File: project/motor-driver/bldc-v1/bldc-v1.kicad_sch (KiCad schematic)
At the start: 51 parts, among them J1 Power, J2 Input, J3 Output, Q1 NMOS, Q2 NMOS, Q3 NMOS, Q4 NMOS, Q5 NMOS, Q6 NMOS, U1 IR2302, U2 IR2302, U3 IR2302

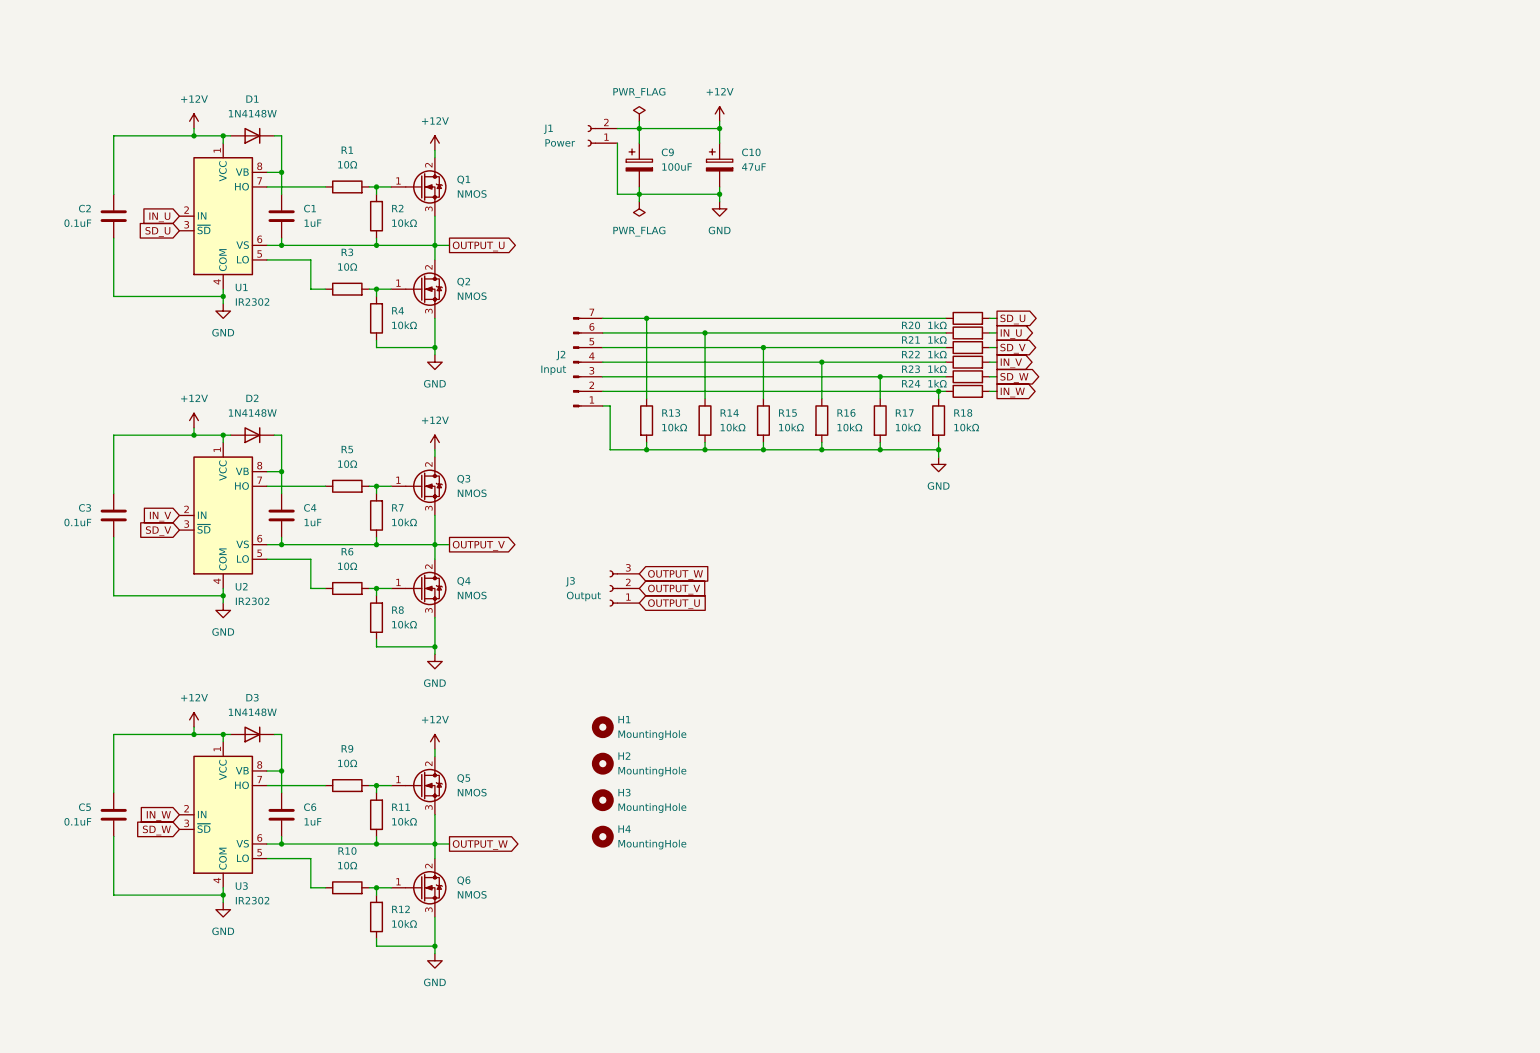
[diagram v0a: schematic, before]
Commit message: 2026/04/22/08:58
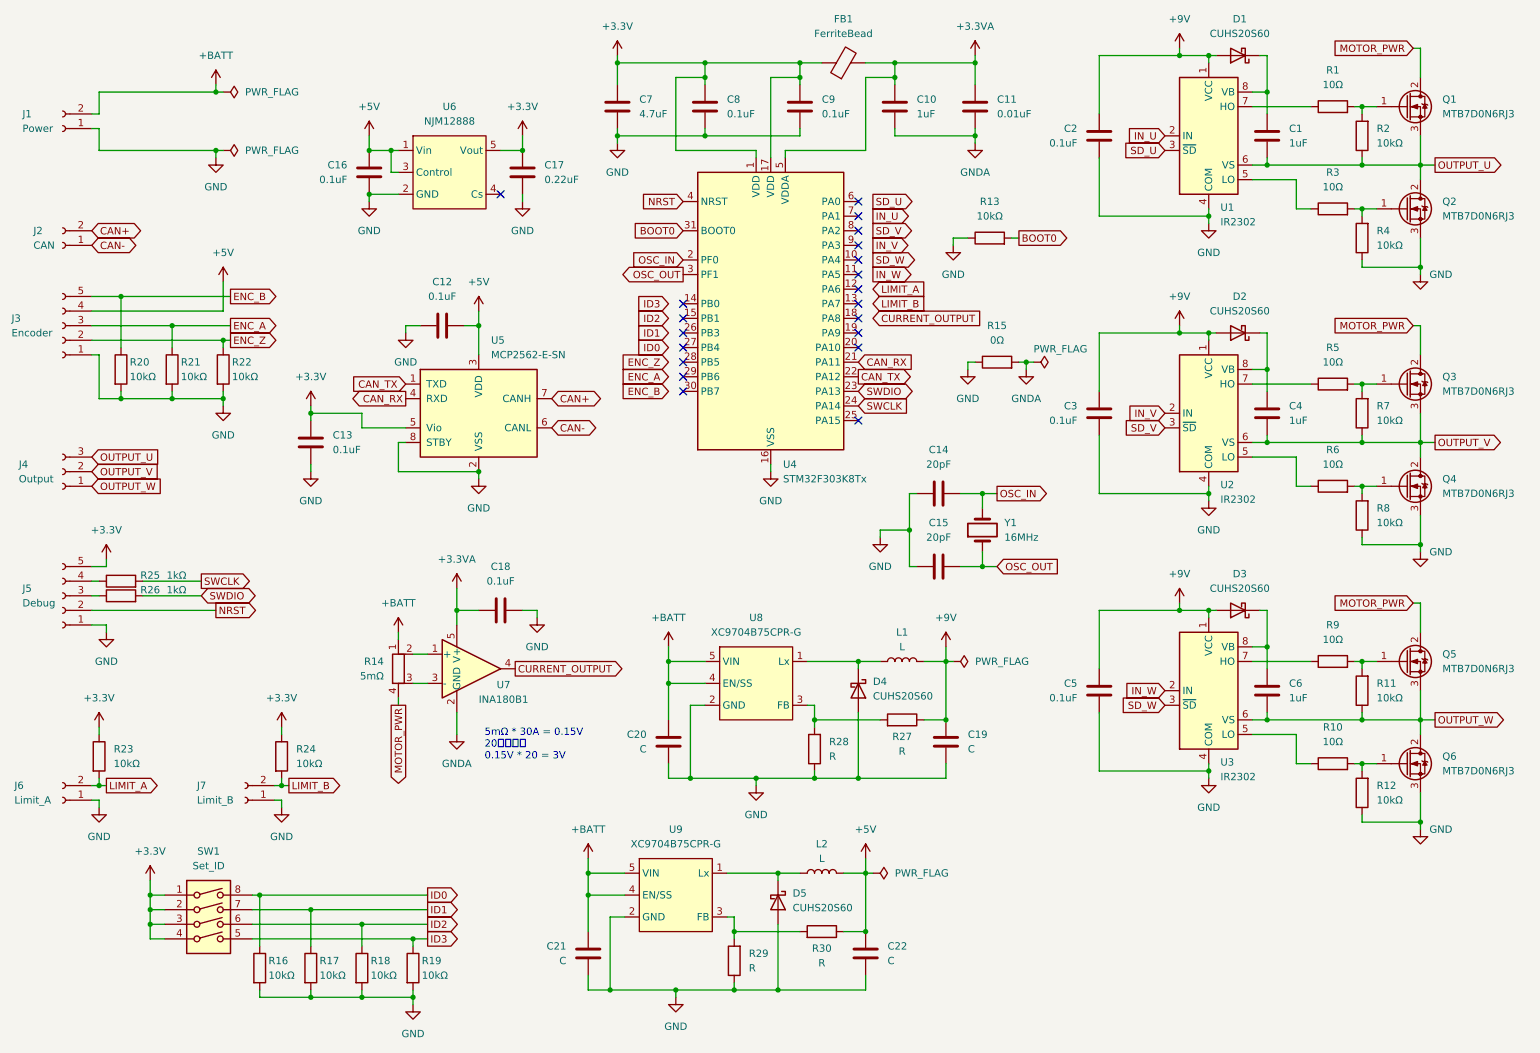
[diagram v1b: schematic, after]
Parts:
- removed C10: 47uF, Capacitor_THT:CP_Radial_D6.3mm_P2.50mm, symbol Device:C_Polarized
- removed C9: 100uF, Capacitor_THT:CP_Radial_D8.0mm_P3.50mm, symbol Device:C_Polarized
- removed D1, D2, D3: 1N4148W, Diode_SMD:D_SOD-123, symbol Diode:1N4148W
- removed H1, H2, H3, H4: MountingHole, MountingHole:MountingHole_3.2mm_M3, symbol Mechanical:MountingHole
- removed J2: Input, Connector_JST:JST_XH_S7B-XH-A_1x07_P2.50mm_Horizontal, symbol Connector:Conn_01x07_Pin
- removed J3: Output, Connector_AMASS:AMASS_MR30PW-FB_1x03_P3.50mm_Horizontal, symbol Connector:Conn_01x03_Socket
- removed R14: 10kΩ, Resistor_SMD:R_0603_1608Metric, symbol Device:R
- added C10: 1uF, symbol Device:C
- added C11: 0.01uF, symbol Device:C
- added C12, C13, C16, C18, C8, C9: 0.1uF, symbol Device:C
- added C14, C15: 20pF, symbol Device:C
- added C17: 0.22uF, symbol Device:C
- added C19, C20, C21, C22: C, symbol Device:C
- added C7: 4.7uF, symbol Device:C
- added D1, D2, D3, D4, D5: CUHS20S60, Diode_SMD:D_SOD-323, symbol Device:D_Schottky
- added FB1: FerriteBead, symbol Device:FerriteBead
- added J2: CAN, symbol Connector:Conn_01x02_Socket
- added J3: Encoder, symbol Connector:Conn_01x05_Socket
- added J4: Output, symbol Connector:Conn_01x03_Socket
- added J5: Debug, symbol Connector:Conn_01x05_Socket
- added J6: Limit_A, symbol Connector:Conn_01x02_Socket
- added J7: Limit_B, symbol Connector:Conn_01x02_Socket
- added L1, L2: L, symbol Device:L
- added R14: 5mΩ, symbol Device:R_Shunt
- added R25, R26: 1kΩ, symbol Device:R
- added R27, R28, R29, R30: R, symbol Device:R
- added SW1: Set_ID, symbol Switch:SW_DIP_x04
- added U4: STM32F303K8Tx, Package_QFP:LQFP-32_7x7mm_P0.8mm, symbol MCU_ST_STM32F3:STM32F303K8Tx
- added U5: MCP2562-E-SN, Package_SO:SOIC-8_3.9x4.9mm_P1.27mm, symbol Interface_CAN_LIN:MCP2562-E-SN
- added U6: NJM12888, Package_TO_SOT_SMD:SOT-23-5, symbol JRC_Regulator_Linear:NJM12888F33
- added U7: INA180B1, Package_TO_SOT_SMD:SOT-23-5, symbol Amplifier_Current:INA180B1
- added U8, U9: XC9704B75CPR-G, Package_TO_SOT_SMD:SOT-89-5, symbol TOREX_Regulator_switching:XC9704B75CPR-G
- added Y1: 16MHz, symbol Device:Crystal
- J1: footprint Connector_AMASS:AMASS_XT30PW-M_1x02_P2.50mm_Horizontal -> (none)
- Q1, Q2, Q3, Q4, Q5, Q6: value NMOS -> MTB7D0N6RJ3
- R13, R16, R17, R18: footprint Resistor_SMD:R_0603_1608Metric -> (none)
- R15: value 10kΩ -> 0Ω; footprint Resistor_SMD:R_0603_1608Metric -> (none)
- R19, R20, R21, R22, R23, R24: value 1kΩ -> 10kΩ; footprint Resistor_SMD:R_0603_1608Metric -> (none)
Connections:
- net GND: now also R13.1, R15.1, R19.2, R20.2, R21.2, R22.2, C12.2, C13.2, C14.1, C15.1, C16.2, C17.2, C18.2, C19.2, C20.2, C21.2, C22.2, C7.2, C8.2, C9.2, D4.2 (A), D5.2 (A), J3.1 (Pin_1), J5.1 (Pin_1), J6.1 (Pin_1), J7.1 (Pin_1), R28.1, R29.1, U4.16 (VSS), U4.32 (VSS), U5.2 (VSS), U5.8 (STBY), U6.2 (GND), U8.2 (GND), U9.2 (GND); no longer R13.2, R15.2
- net IN_U: no longer R20.2
- net IN_V: no longer R22.2
- net IN_W: no longer R24.2
- net OUTPUT_U: now also J4.3 (Pin_3)
- net OUTPUT_V: now also J4.2 (Pin_2)
- net OUTPUT_W: now also J4.1 (Pin_1)
- net SD_U: no longer R19.2
- net SD_V: no longer R21.2
- net SD_W: no longer R23.2
- net ENC_B: now reaches R20.1
- net ENC_B: now also J3.5 (Pin_5)
- net at C1.1, U1.8 (VB): now also D1.1 (K)
- net at C4.1, U2.8 (VB): now also D2.1 (K)
- net at C6.1, U3.8 (VB): now also D3.1 (K)
- net +3.3V: now reaches R23.1
- net +3.3V: now also R24.1, C13.1, C17.1, C7.1, C8.1, C9.1, FB1.1, J5.5 (Pin_5), SW1.1, SW1.2, SW1.3, SW1.4, U4.1 (VDD), U4.17 (VDD), U5.5 (Vio), U6.5 (Vout); no longer R17.1
- net ID2: now reaches R18.1
- net ID2: now also SW1.6; no longer R24.1
- net ENC_A: now reaches R21.1
- net ENC_A: now also J3.3 (Pin_3); no longer R15.1
- net ENC_Z: now reaches R22.1
- net ENC_Z: now also J3.2 (Pin_2); no longer R16.1
- net ID3: now reaches R19.1
- net ID3: now also SW1.5; no longer R13.1
- net +12V renamed +9V
- net +9V: now also C19.1, D1.2 (A), D2.2 (A), D3.2 (A), L1.2, R27.1; no longer J1.2 (Pin_2), Q1.2 (D), Q3.2 (D), Q5.2 (D)
- new net: R29.2, R30.2, U9.3 (FB)
- new net: R14.2, U7.1 (+)
- new net: R14.3, U7.3 (-)
- new net: D4.1 (K), L1.1, U8.1 (Lx)
- new net: R27.2, R28.2, U8.3 (FB)
- new net: D5.1 (K), L2.1, U9.1 (Lx)
- new net: J5.4 (Pin_4), R25.1
- new net: J5.3 (Pin_3), R26.1
- new net +3.3VA: C10.1, C11.1, C18.1, FB1.2, U4.5 (VDDA), U7.5 (V+)
- new net +5V: C12.1, C16.1, C22.1, J3.4 (Pin_4), L2.2, R30.1, U5.3 (VDD), U6.1 (Vin), U6.3 (Control)
- new net +BATT: C20.1, C21.1, J1.2 (Pin_2), R14.1, U8.4 (EN/SS), U8.5 (VIN), U9.4 (EN/SS), U9.5 (VIN)
- new net BOOT0: R13.2, U4.31 (BOOT0)
- new net CAN+: J2.2 (Pin_2), U5.7 (CANH)
- new net CAN-: J2.1 (Pin_1), U5.6 (CANL)
- new net CAN_RX: U4.21 (PA11), U5.4 (RXD)
- new net CAN_TX: U4.22 (PA12), U5.1 (TXD)
- new net CURRENT_OUTPUT: U7.4
- new net GNDA: C10.2, C11.2, R15.2, U7.2 (GND)
- new net ID0: R16.1, SW1.8
- new net ID1: R17.1, SW1.7
- new net LIMIT_A: J6.2 (Pin_2), R23.2
- new net LIMIT_B: J7.2 (Pin_2), R24.2
- new net MOTOR_PWR: Q1.2 (D), Q3.2 (D), Q5.2 (D), R14.4
- new net NRST: J5.2 (Pin_2), U4.4 (NRST)
- new net OSC_IN: C14.2, U4.2 (PF0), Y1.2
- new net OSC_OUT: C15.2, U4.3 (PF1), Y1.1
- new net SWCLK: R25.2, U4.24 (PA14)
- new net SWDIO: R26.2, U4.23 (PA13)
- no-connect marks 0 -> 20
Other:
- note added: "5mΩ * 30A = 0.15V 20倍なので 0.15V * 20 = 3V"
- moved on the sheet: C1, C2, C3, C4, C5, C6, Q1, Q2, Q3, Q4, Q5, Q6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
